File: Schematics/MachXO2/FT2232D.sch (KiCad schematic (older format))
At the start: 44 parts, among them J3 USB_B_Micro, U2 FT2232D, U4 93C56, X2 6.00MHz

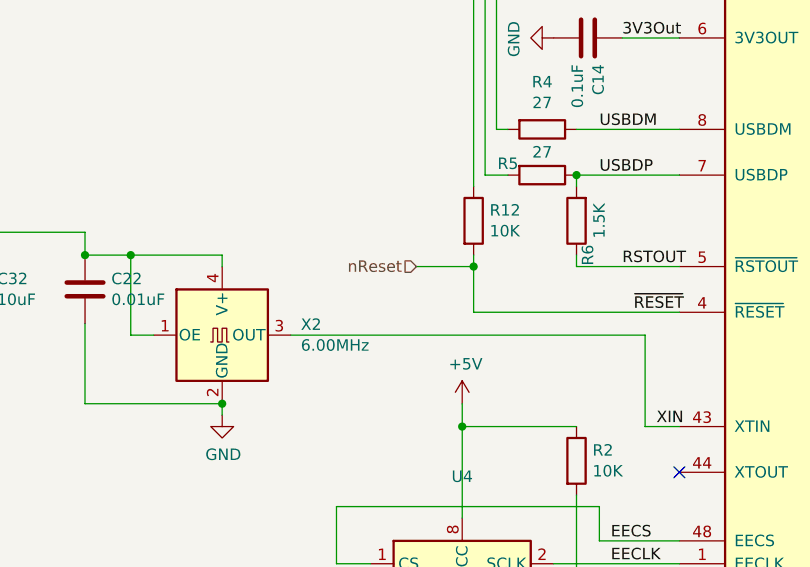
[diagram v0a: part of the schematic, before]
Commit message: Update Gerber Data to RevA5
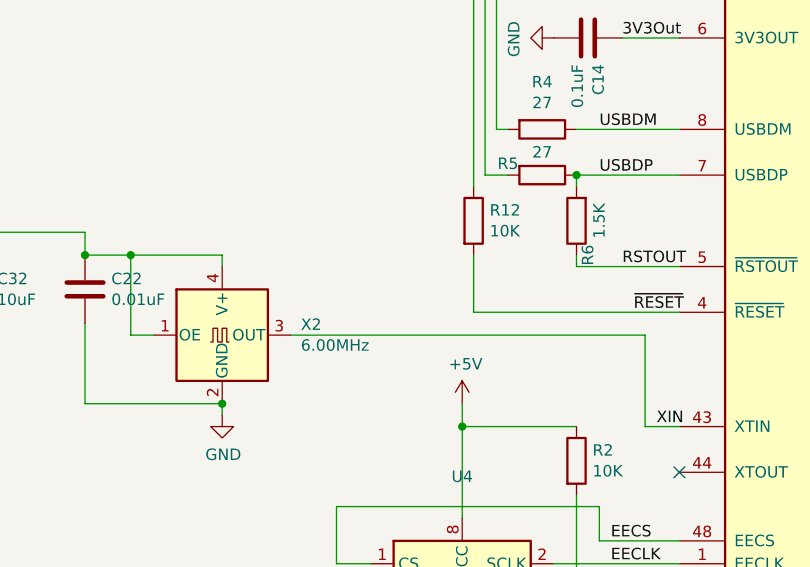
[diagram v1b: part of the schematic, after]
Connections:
- net nReset renamed ~RESET
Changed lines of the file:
@@
 Wire Wire Line
 	4750 5850 5500 5850
-Text HLabel 3750 3550 0    50   Input ~ 0
-nReset
 $Comp
 L CPU2908CLocal:R R1
@@
 	7900 1700 7700 1700
 $Comp
-L Memory_EEPROM:93CxxA U4
-U 1 1 5DC82A54
-P 3950 4950
-F 0 "U4" H 3950 5431 50  0000 C CNN
-F 1 "93C56" H 3700 4650 50  0000 C CNN
-F 2 "Housings_SOIC:SOIC-8_3.9x4.9mm_Pitch1.27mm" H 3950 4950 50  0001 C CNN
-F 3 "http://ww1.microchip.com/downloads/en/DeviceDoc/20001749K.pdf" H 3950 4950 50  0001 C CNN
-	1    3950 4950
-	1    0    0    -1
-$EndComp
-$Comp
 L power:GND #PWR0104
 U 1 1 5DC86D51
@@
 	4350 4850 4900 4850
 Wire Wire Line
-	3400 4850 3550 4850
-Wire Wire Line
 	4350 4950 4850 4950
 Wire Wire Line
@@
 	4450 4550 4450 5050
 Wire Wire Line
-	4550 4600 3400 4600
-Wire Wire Line
 	4550 4600 4550 4750
-Wire Wire Line
-	3400 4600 3400 4850
 $Comp
 L CPU2908CLocal:R R3
@@
 	4500 5050 4450 5050
 Connection ~ 4450 5050
-$Comp
-L o2_breakout-rescue:SG-8002CA-Oscillator X?
-U 1 1 5DC12BA3
-P 2900 3850
-AR Path="/5DC12BA3" Ref="X?"  Part="1"
-AR Path="/5E6A6650/5DC12BA3" Ref="X2"  Part="1"
-F 0 "X2" H 3244 3896 50  0000 L CNN
-F 1 "6.00MHz" H 3244 3805 50  0000 L CNN
-F 2 "Oscillators:Oscillator_SMD_SeikoEpson_SG8002LB-4pin_5.0x3.2mm_HandSoldering" H 3600 3500 50  0001 C CNN
-F 3 "https://support.epson.biz/td/api/doc_check.php?mode=dl&lang=en&Parts=SG-8002DC" H 2800 3850 50  0001 C CNN
-	1    2900 3850
-	1    0    0    -1
-$EndComp
-Wire Wire Line
-	3200 3850 4750 3850
 Wire Wire Line
 	4750 3850 4750 4250
@@
 	4750 4250 4900 4250
 Wire Wire Line
-	2900 4150 2900 4200
-$Comp
-L power:GND #PWR015
-U 1 1 5DC1A4C5
-P 2900 4200
-F 0 "#PWR015" H 2900 3950 50  0001 C CNN
-F 1 "GND" H 2905 4027 50  0000 C CNN
-F 2 "" H 2900 4200 50  0001 C CNN
-F 3 "" H 2900 4200 50  0001 C CNN
-	1    2900 4200
-	1    0    0    -1
-$EndComp
-Wire Wire Line
 	2600 3850 2500 3850
 Wire Wire Line
 	2500 3850 2500 3500
-Wire Wire Line
-	2500 3500 2900 3500
 Wire Wire Line
 	4450 3150 4900 3150
@@
 	1    0    0    -1
 $EndComp
-Wire Wire Line
-	2900 3500 2900 3550
 $Comp
 L Device:C C22
@@
 Wire Wire Line
 	2300 3500 2500 3500
-Connection ~ 2500 3500
 Wire Wire Line
 	2300 3800 2300 4150
-Wire Wire Line
-	2300 4150 2900 4150
-Connection ~ 2900 4150
 Wire Wire Line
 	3950 5250 3950 5350
@@
 	4650 2550 4900 2550
 Wire Wire Line
-	4000 3500 4000 3550
-Wire Wire Line
-	3750 3550 4000 3550
-Connection ~ 4000 3550
-Wire Wire Line
-	4000 3550 4000 3750
-Wire Wire Line
 	4000 3750 4900 3750
 Wire Wire Line
@@
 Wire Wire Line
 	4000 1500 5400 1500
+Wire Wire Line
+	2300 4150 2900 4150
+Wire Wire Line
+	2900 3500 2900 3550
+Connection ~ 2500 3500
+Wire Wire Line
+	2500 3500 2900 3500
+$Comp
+L power:GND #PWR015
+U 1 1 5DC1A4C5
+P 2900 4200
+F 0 "#PWR015" H 2900 3950 50  0001 C CNN
+F 1 "GND" H 2905 4027 50  0000 C CNN
+F 2 "" H 2900 4200 50  0001 C CNN
+F 3 "" H 2900 4200 50  0001 C CNN
+	1    2900 4200
+	1    0    0    -1
+$EndComp
+Wire Wire Line
+	2900 4150 2900 4200
+Wire Wire Line
+	3200 3850 4750 3850
+Connection ~ 2900 4150
+$Comp
+L o2_breakout-rescue:SG-8002CA-Oscillator X?
+U 1 1 5DC12BA3
+P 2900 3850
+AR Path="/5DC12BA3" Ref="X?"  Part="1"
+AR Path="/5E6A6650/5DC12BA3" Ref="X2"  Part="1"
+F 0 "X2" H 3244 3896 50  0000 L CNN
+F 1 "6.00MHz" H 3244 3805 50  0000 L CNN
+F 2 "Oscillators:Oscillator_SMD_SeikoEpson_SG8002LB-4pin_5.0x3.2mm_HandSoldering" H 3600 3500 50  0001 C CNN
+F 3 "https://support.epson.biz/td/api/doc_check.php?mode=dl&lang=en&Parts=SG-8002DC" H 2800 3850 50  0001 C CNN
+	1    2900 3850
+	1    0    0    -1
+$EndComp
+Wire Wire Line
+	3400 4600 3400 4850
+Wire Wire Line
+	4550 4600 3400 4600
+Wire Wire Line
+	3400 4850 3550 4850
+$Comp
+L Memory_EEPROM:93CxxA U4
+U 1 1 5DC82A54
+P 3950 4950
+F 0 "U4" H 3950 5431 50  0000 C CNN
+F 1 "93C56" H 3700 4650 50  0000 C CNN
+F 2 "Housings_SOIC:SOIC-8_3.9x4.9mm_Pitch1.27mm" H 3950 4950 50  0001 C CNN
+F 3 "http://ww1.microchip.com/downloads/en/DeviceDoc/20001749K.pdf" H 3950 4950 50  0001 C CNN
+	1    3950 4950
+	1    0    0    -1
+$EndComp
+Wire Wire Line
+	4000 3500 4000 3750
 $EndSCHEMATC
